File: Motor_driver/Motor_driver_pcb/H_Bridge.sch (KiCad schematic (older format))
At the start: 18 parts, among them Q1 2N2222, Q2 IRF9540N, Q3 IRF540N, Q4 IRF9540N, Q5 IRF540N, Q6 2N2222

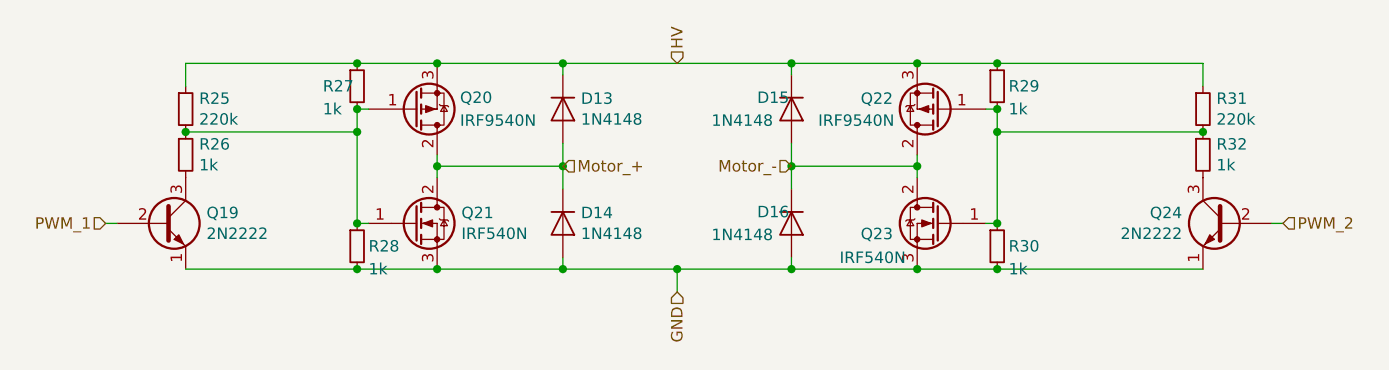
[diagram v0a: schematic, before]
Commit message: add final parts and working code
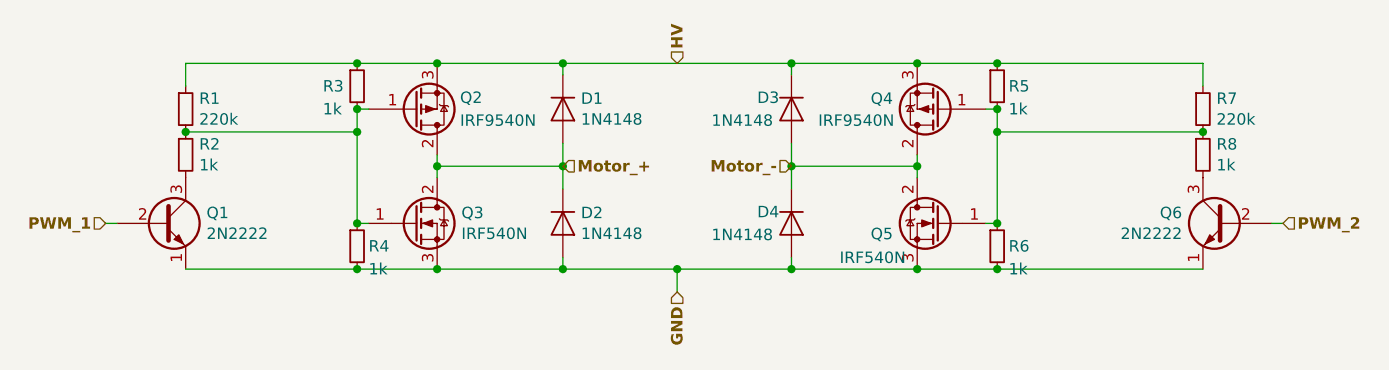
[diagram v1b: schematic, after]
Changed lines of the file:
@@
 AR Path="/5CA1B151/5C9E42AA" Ref="Q15"  Part="1"
 AR Path="/5CA227B5/5C9E42AA" Ref="Q21"  Part="1"
-F 0 "Q21" H 4056 3046 50  0000 L CNN
+F 0 "Q3" H 4056 3046 50  0000 L CNN
 F 1 "IRF540N" H 4056 2955 50  0000 L CNN
 F 2 "Package_TO_SOT_THT:TO-220-3_Vertical" H 4100 2925 50  0001 L CIN
@@
 AR Path="/5CA1B151/5C9E4811" Ref="Q14"  Part="1"
 AR Path="/5CA227B5/5C9E4811" Ref="Q20"  Part="1"
-F 0 "Q20" H 4050 2450 50  0000 L CNN
+F 0 "Q2" H 4050 2450 50  0000 L CNN
 F 1 "IRF9540N" H 4050 2550 50  0000 L CNN
 F 2 "Package_TO_SOT_THT:TO-220-3_Vertical" H 4050 2425 50  0001 L CIN
@@
 AR Path="/5CA1B151/5C9E549E" Ref="D9"  Part="1"
 AR Path="/5CA227B5/5C9E549E" Ref="D13"  Part="1"
-F 0 "D13" V 4454 2579 50  0000 L CNN
+F 0 "D1" V 4454 2579 50  0000 L CNN
 F 1 "1N4148" V 4545 2579 50  0000 L CNN
 F 2 "Diode_THT:D_DO-35_SOD27_P7.62mm_Horizontal" H 4500 2325 50  0001 C CNN
@@
 AR Path="/5CA1B151/5C9E5F82" Ref="D10"  Part="1"
 AR Path="/5CA227B5/5C9E5F82" Ref="D14"  Part="1"
-F 0 "D14" V 4454 3079 50  0000 L CNN
+F 0 "D2" V 4454 3079 50  0000 L CNN
 F 1 "1N4148" V 4545 3079 50  0000 L CNN
 F 2 "Diode_THT:D_DO-35_SOD27_P7.62mm_Horizontal" H 4500 2825 50  0001 C CNN
@@
 AR Path="/5CA1B151/5C9E6D79" Ref="Q16"  Part="1"
 AR Path="/5CA227B5/5C9E6D79" Ref="Q22"  Part="1"
-F 0 "Q22" H 6356 2454 50  0000 L CNN
+F 0 "Q4" H 6356 2454 50  0000 L CNN
 F 1 "IRF9540N" H 6350 2550 50  0000 L CNN
 F 2 "Package_TO_SOT_THT:TO-220-3_Vertical" H 6350 2425 50  0001 L CIN
@@
 AR Path="/5CA1B151/5C9E8C92" Ref="Q17"  Part="1"
 AR Path="/5CA227B5/5C9E8C92" Ref="Q23"  Part="1"
-F 0 "Q23" H 6356 2954 50  0000 L CNN
+F 0 "Q5" H 6356 2954 50  0000 L CNN
 F 1 "IRF540N" H 6300 2850 50  0000 L CNN
 F 2 "Package_TO_SOT_THT:TO-220-3_Vertical" H 6400 2925 50  0001 L CIN
@@
 AR Path="/5CA1B151/5C9EAA23" Ref="D11"  Part="1"
 AR Path="/5CA227B5/5C9EAA23" Ref="D15"  Part="1"
-F 0 "D15" V 5450 2350 50  0000 L CNN
+F 0 "D3" V 5450 2350 50  0000 L CNN
 F 1 "1N4148" V 5550 2150 50  0000 L CNN
 F 2 "Diode_THT:D_DO-35_SOD27_P7.62mm_Horizontal" H 5500 2325 50  0001 C CNN
@@
 AR Path="/5CA1B151/5C9EC3FB" Ref="D12"  Part="1"
 AR Path="/5CA227B5/5C9EC3FB" Ref="D16"  Part="1"
-F 0 "D16" V 5450 2850 50  0000 L CNN
+F 0 "D4" V 5450 2850 50  0000 L CNN
 F 1 "1N4148" V 5550 2650 50  0000 L CNN
 F 2 "Diode_THT:D_DO-35_SOD27_P7.62mm_Horizontal" H 5500 2825 50  0001 C CNN
@@
 Wire Wire Line
 	4500 3200 5000 3200
-Text HLabel 2500 3000 0    50   Input ~ 0
+Text HLabel 2500 3000 0    50   Input ~ 10
 PWM_1
-Text HLabel 7650 3000 2    50   Input ~ 0
+Text HLabel 7650 3000 2    50   Input ~ 10
 PWM_2
-Text HLabel 5000 3300 3    50   Input ~ 0
+Text HLabel 5000 3300 3    50   Input ~ 10
 GND
 Wire Wire Line
@@
 Connection ~ 4500 2300
 Connection ~ 5500 2300
-Text HLabel 5000 2300 1    50   Input ~ 0
+Text HLabel 5000 2300 1    50   Input ~ 10
 HV
-Text HLabel 4500 2750 2    50   Input ~ 0
+Text HLabel 4500 2750 2    50   Input ~ 10
 Motor_+
-Text HLabel 5500 2750 0    50   Input ~ 0
+Text HLabel 5500 2750 0    50   Input ~ 10
 Motor_-
 $Comp
@@
 AR Path="/5CA1B151/5CA04B0F" Ref="R21"  Part="1"
 AR Path="/5CA227B5/5CA04B0F" Ref="R29"  Part="1"
-F 0 "R29" H 6450 2400 50  0000 L CNN
+F 0 "R5" H 6450 2400 50  0000 L CNN
 F 1 "1k" H 6450 2300 50  0000 L CNN
 F 2 "Resistor_SMD:R_0805_2012Metric_Pad1.15x1.40mm_HandSolder" H 6400 2400 50  0001 C CNN
@@
 AR Path="/5CA1B151/5CA04F40" Ref="R22"  Part="1"
 AR Path="/5CA227B5/5CA04F40" Ref="R30"  Part="1"
-F 0 "R30" H 6450 3100 50  0000 L CNN
+F 0 "R6" H 6450 3100 50  0000 L CNN
 F 1 "1k" H 6450 3000 50  0000 L CNN
 F 2 "Resistor_SMD:R_0805_2012Metric_Pad1.15x1.40mm_HandSolder" H 6400 3100 50  0001 C CNN
@@
 AR Path="/5CA1B151/5CA0523E" Ref="R20"  Part="1"
 AR Path="/5CA227B5/5CA0523E" Ref="R28"  Part="1"
-F 0 "R28" H 3650 3100 50  0000 L CNN
+F 0 "R4" H 3650 3100 50  0000 L CNN
 F 1 "1k" H 3650 3000 50  0000 L CNN
 F 2 "Resistor_SMD:R_0805_2012Metric_Pad1.15x1.40mm_HandSolder" H 3600 3100 50  0001 C CNN
@@
 AR Path="/5CA1B151/5CA057A9" Ref="R19"  Part="1"
 AR Path="/5CA227B5/5CA057A9" Ref="R27"  Part="1"
-F 0 "R27" H 3450 2400 50  0000 L CNN
+F 0 "R3" H 3450 2400 50  0000 L CNN
 F 1 "1k" H 3450 2300 50  0000 L CNN
 F 2 "Resistor_SMD:R_0805_2012Metric_Pad1.15x1.40mm_HandSolder" H 3600 2400 50  0001 C CNN
@@
 AR Path="/5CA1B151/5CABFFC4" Ref="R18"  Part="1"
 AR Path="/5CA227B5/5CABFFC4" Ref="R26"  Part="1"
-F 0 "R26" H 2909 2746 50  0000 L CNN
+F 0 "R2" H 2909 2746 50  0000 L CNN
 F 1 "1k" H 2909 2655 50  0000 L CNN
 F 2 "Resistor_SMD:R_0805_2012Metric_Pad1.15x1.40mm_HandSolder" H 2850 2700 50  0001 C CNN
@@
 AR Path="/5CA1B151/5CAC04F6" Ref="R17"  Part="1"
 AR Path="/5CA227B5/5CAC04F6" Ref="R25"  Part="1"
-F 0 "R25" H 2909 2546 50  0000 L CNN
+F 0 "R1" H 2909 2546 50  0000 L CNN
 F 1 "220k" H 2909 2455 50  0000 L CNN
 F 2 "Resistor_SMD:R_0805_2012Metric_Pad1.15x1.40mm_HandSolder" H 2850 2500 50  0001 C CNN
@@
 AR Path="/5CA1B151/5CBAE7DE" Ref="R24"  Part="1"
 AR Path="/5CA227B5/5CBAE7DE" Ref="R32"  Part="1"
-F 0 "R32" H 7359 2746 50  0000 L CNN
+F 0 "R8" H 7359 2746 50  0000 L CNN
 F 1 "1k" H 7359 2655 50  0000 L CNN
 F 2 "Resistor_SMD:R_0805_2012Metric_Pad1.15x1.40mm_HandSolder" H 7300 2700 50  0001 C CNN
@@
 AR Path="/5CA1B151/5CBAE7E4" Ref="R23"  Part="1"
 AR Path="/5CA227B5/5CBAE7E4" Ref="R31"  Part="1"
-F 0 "R31" H 7359 2546 50  0000 L CNN
+F 0 "R7" H 7359 2546 50  0000 L CNN
 F 1 "220k" H 7359 2455 50  0000 L CNN
 F 2 "Resistor_SMD:R_0805_2012Metric_Pad1.15x1.40mm_HandSolder" H 7300 2500 50  0001 C CNN
@@
 AR Path="/5CA1B151/5CC73221" Ref="Q13"  Part="1"
 AR Path="/5CA227B5/5CC73221" Ref="Q19"  Part="1"
-F 0 "Q19" H 2941 3046 50  0000 L CNN
+F 0 "Q1" H 2941 3046 50  0000 L CNN
 F 1 "2N2222" H 2941 2955 50  0000 L CNN
 F 2 "Package_TO_SOT_THT:TO-92" H 2950 3100 50  0001 C CNN
@@
 AR Path="/5CA1B151/5CC746B3" Ref="Q18"  Part="1"
 AR Path="/5CA227B5/5CC746B3" Ref="Q24"  Part="1"
-F 0 "Q24" H 7591 3046 50  0000 L CNN
+F 0 "Q6" H 7591 3046 50  0000 L CNN
 F 1 "2N2222" H 7591 2955 50  0000 L CNN
 F 2 "Package_TO_SOT_THT:TO-92" H 7600 3100 50  0001 C CNN
